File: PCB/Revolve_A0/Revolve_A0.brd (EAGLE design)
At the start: 100 x 100 mm, 386 parts, among them IC29 LAN8710A, IC30 MTFC2GMDEA, IC6 74AHC1G126DCK, IC7 74AHC1G126DCK, J2 4P-2.0, J3 4P-2.0, Q1 AON6758, Q10 DMC2038LVT, Q11 DMC2038LVT, Q13 DMC2038LVT, Q14 DMC2038LVT, Q2 AON6758, Q3 AON6758, Q8 AON6758, Q9 MMBT2907, U1 OSD3358-512M-BSM, U10 TPD4S012_DRY_6, U11 SN74AHC595PW, U13 INA199A1DCKR, U19 CD4050BD, U2 TUSB2046BIRHBT, U3 TPS2061D, U4 TPD4S012_DRY_6_P1_P, U5 UA78L05ACD, U6 TPD4S012_DRY_6_P1_P, U7 TLVH431, U8 TPD4S012_DRY_6_P1_P, U9 TPD4S012_DRY_6_P1_P, X1 22-05-7038-03, X10 22-05-7038-03, X11 22-05-7038-03, X12 22-05-7048-04, X13 22-05-7038-03, X14 22-05-7048-04, X15 22-05-7048-04, X16 22-05-7048-04, X17 22-05-7048-04, X18 22-05-7048-04, X19 22-05-7038-03, X2 MSTBA4, X20 MSTBA4, X21 MSTBA2, X22 22-05-7038-03, X24 HDMI4, X25 22-05-7048-04, X26 MSTBA2, X29 22-05-7038-03, X3 MSTBA2, X4 22-05-7028-02, X5 22-05-7028-02, X6 22-05-7028-02, X7 22-05-7038-03, X8 22-05-7038-03, X9 22-05-7028-02, Y1 25MHz, Y2 25MHz, Y4 6 MHz

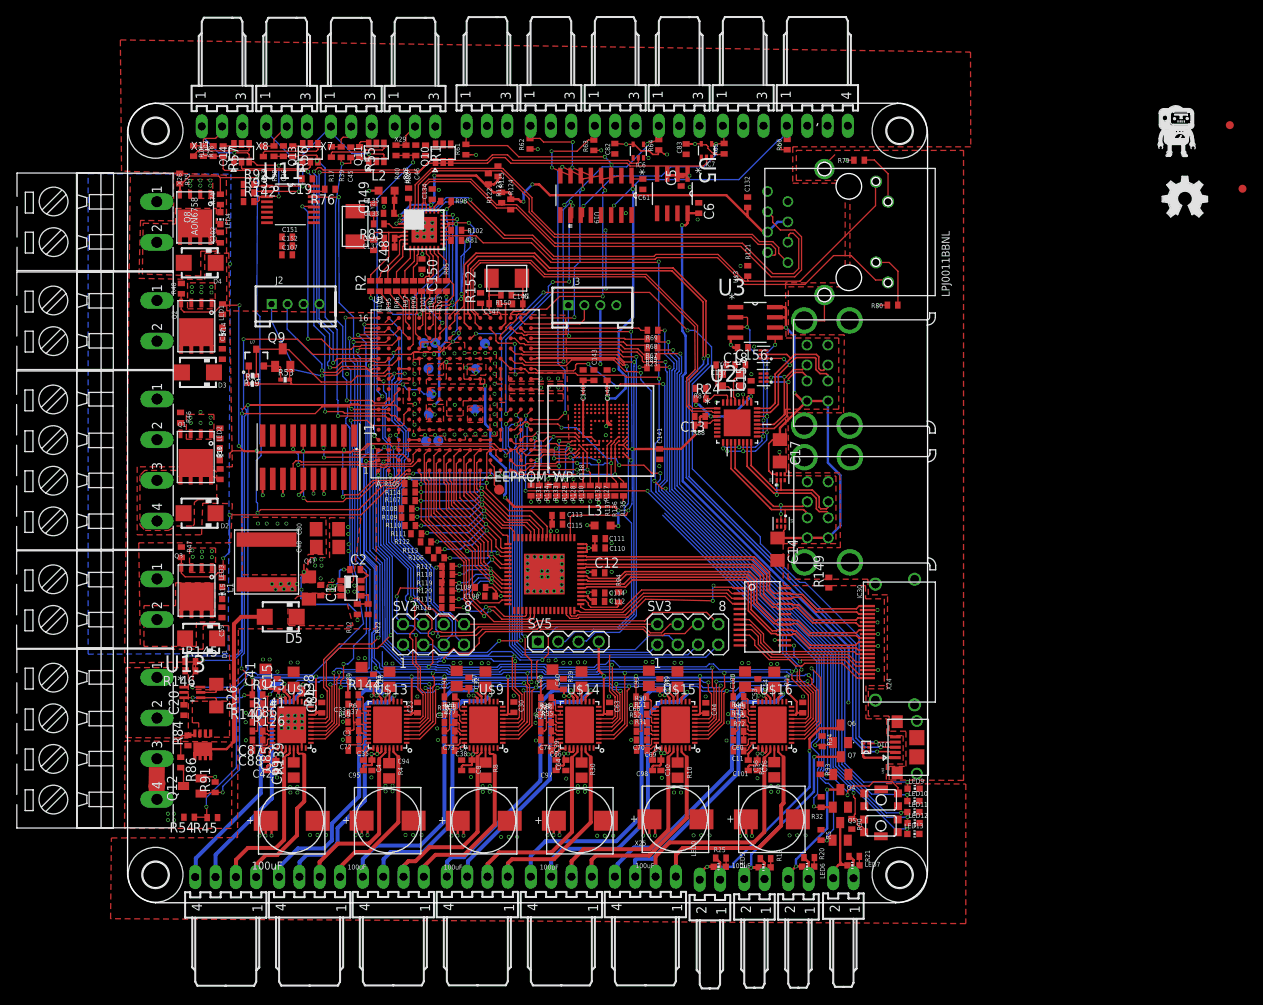
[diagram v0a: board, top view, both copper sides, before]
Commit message: Working on DRC errors
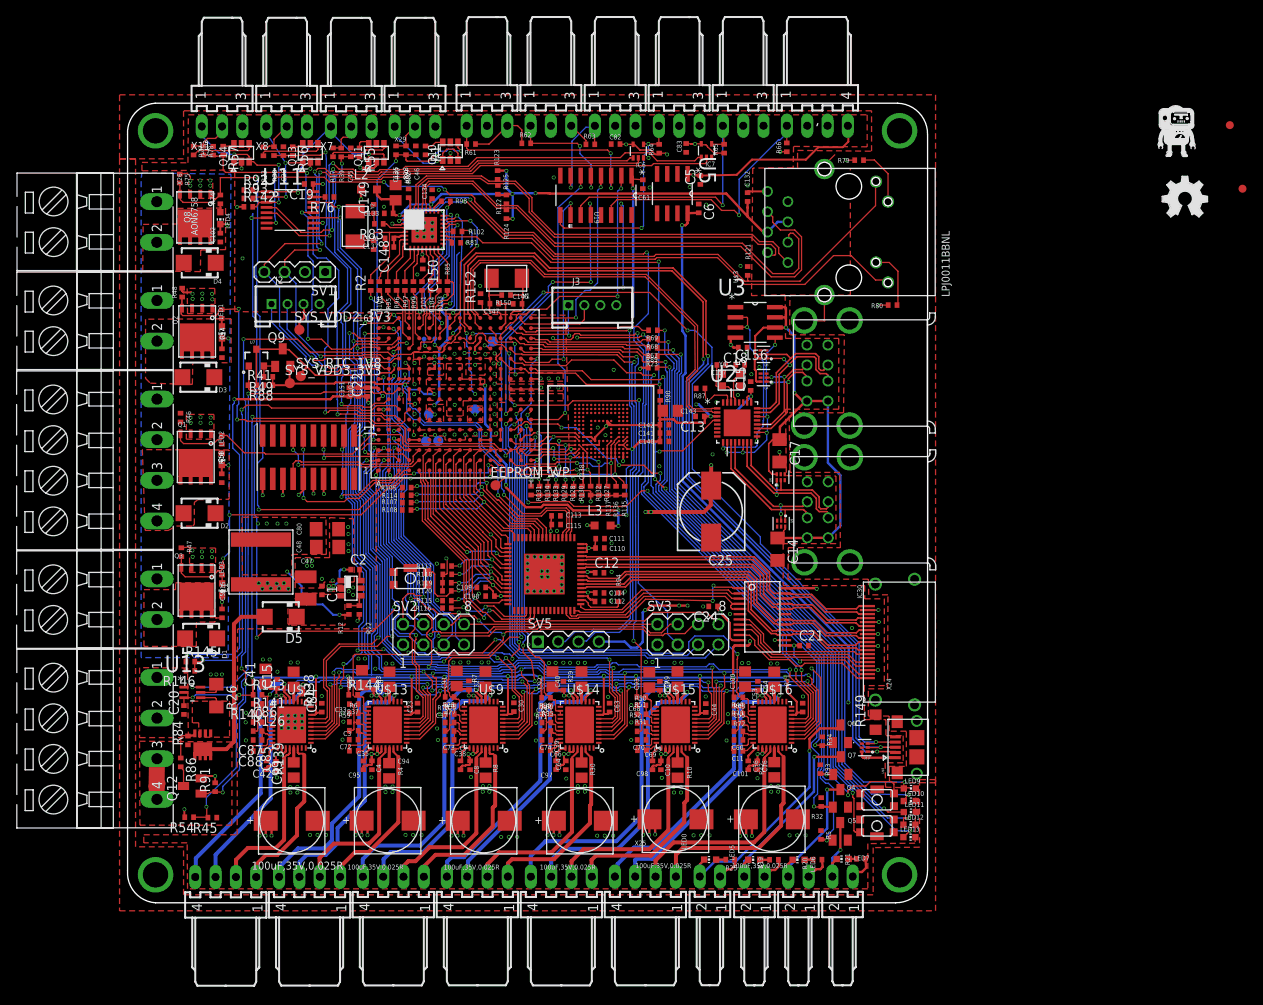
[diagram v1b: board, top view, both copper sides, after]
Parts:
- removed C152: 0.001uF, rcl:C0402
- removed H1, H2, H3, H4: MOUNT-HOLE3.2, holes:3,2
- removed R106, R109, R110, R111, R112, R113: 100K,1%, rcl:R0402
- removed R24: 0R,DNI, rcl:R0402
- removed R53: 499, OSD3358-SM-RED Platform:R0402
- added C21, C24: 0.1uF, rcl:C0402
- added C22: 4.7nF, rcl:C0402
- added C25: (no value), rcl:150CLZ-0810
- added MGT1, MGT2, MGT3, MGT4: MOUNTING_HOLE, OSD3358-SM-RED Platform:MOUNTING_HOLE
- added S1: KRM_TACT_SWITCH, Manga_custom:KMR
- added SV1: (no value), con-lstb:MA04-1
- C101, C42, C94, C95, C97, C98: value 100uF -> 100uF,35V,0.025R
- C132: value 0.022uF -> 22nF
- C135, C143: value 10uF -> 10uF,3.3V; device rcl:C0402 -> rcl:C0805
- C47: value 10uF -> 10uF,35V; device rcl:C1206 -> rcl:C1210
- L1: value 33uH -> 15uH
- R1, R121, R140, R141, R27, R31, R35, R37, R38, R39, R40, R43, R50, R55, R56, R57, R58, R6, R60, R73, R78, R81, R88: value 10K -> 10K,1%
- R122, R123, R124, R125: value 49.1, 1% -> 49.9,1%
- R127, R128, R129, R130, R131, R132, R133, R134, R135, R136, R137, R14, R142, R143, R144, R15, R16, R19, R20, R21, R23, R25, R28, R32, R33, R34, R36, R44, R46, R47, R48, R5, R51, R54, R61, R62, R63, R64, R65, R66, R67, R68, R69, R74, R75, R76, R87, R89, R91, R92, R93: value 4.7K -> 4.7K,1%
- R13, R17, R18, R77: value 4K7, 1% -> 4.7K,1%
- R149: value 0.1,5% -> 0.1R; device rcl:R0402 -> rcl:R0805
- R41: value 10K, 1% -> 40.2K,1%; device OSD3358-SM-RED Platform:R0402 -> rcl:R0402
- R49: value 40.2K, 1% -> 470; device OSD3358-SM-RED Platform:R0402 -> rcl:R0402
- R83: value 10 -> 10,1%
- SV2, SV3: value (none) -> DNI
- U10: value TPD4S012_DRY_6 -> TPD4S012_DRY_6_P1_P; device BeagleBone_Blue:DRY6 -> OSD3358-SM-RED Platform:DRY6
- VDDS_PLL, VDD_MPU: value TPB1,27 -> TPTP06R; device testpad:B1,27 -> testpad:TP06R
- moved R90 58.6 mm to (66.6, 63.4)
- moved R88 54.2 mm to (17.6, 64.7)
- moved SYS_RTC_1V8 21.9 mm to (21.7, 65.8), flipped to the top
- moved C151 20.9 mm to (27.7, 63.9), turned to 90 degrees
- moved C107 19.3 mm to (28.9, 63.9), turned to 90 degrees
- moved R149 18.4 mm to (93.5, 22.6)
- moved SYS_VDD3_3V3 17.7 mm to (20.3, 65.0), flipped to the top
- moved SYS_VDD2_3V3 16.9 mm to (21.5, 71.6), flipped to the top
- moved C140 13.1 mm to (67.1, 57.7), turned to 0 degrees
- moved C143 10.5 mm to (67.9, 61.5), turned to 0 degrees
- moved C142 9.47 mm to (67.1, 59.8), turned to 0 degrees
- moved C141 2.70 mm to (67.1, 58.7), turned to 0 degrees
- moved C5 2.40 mm to (71.6, 90.3)
- moved L2 2.21 mm to (30.2, 89.2)
- moved R49 2.01 mm to (17.6, 65.8)
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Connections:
- removed net FAULT_B: SV2.1, U1.T12
- removed net FAULT_C: SV3.1, U1.R5
- removed net PMIC_SCL: U1.C10, U1.D10
- removed net PMIC_SDA: U1.C11, U1.D11
- removed net TK_H: U1.C8
- removed net TRSRTN: J1.2
- removed net UNUSED_1: U1.J14
- removed net USB1_DRVVBUS: U1.M14
- removed net USB_RESET: R88.1, U2.4
- removed net VDD_3V3B: R90.1
- new net PMIC_MUX: U1.C8, U1.N13
- net +5V: no longer C18.2, C19.1, C82.1, C83.1, IC6.5, IC7.5, R61.2, R62.2, R63.2, R64.2, R65.2, R66.2, U$18.P$11, U11.10, U11.16, U3.4, X1.3, X10.3, X12.3, X13.3, X19.3, X22.3
- net CGND: now also MGT1.P$1, MGT2.P$1, MGT3.P$1, MGT4.P$1
- net CLKOUT2_48MHZ: no longer U2.27
- net DVI_+5V: now also C21.1
- net ENABLE_B: now also U11.6; no longer U1.T7
- net ENABLE_C: now also U11.7; no longer U1.R7
- net FAULT_A: now also U1.R5
- net FAULT_E: now also U1.T7
- net FAULT_H: now also U1.J14
- net FAULT_Y: now also U1.R7
- net FAULT_Z: now also U1.T12
- net GND: now also C21.2, C24.2, C25.-, R117.2, S1.2, SV1.1, SV2.1, SV3.1; no longer R106.1, R109.1, R110.1, R111.1, R112.1, R113.1
- net GNDA_ADC: now also C22.2; no longer C152.2
- net HDMI_HPD: now also U$18.P$5
- net I2C0_SCL: now also U1.C10, U1.D10
- net I2C0_SDA: now also U1.C11, U1.D11
- net LCD_D10: no longer R110.2
- net LCD_D11: no longer R109.2
- net LCD_D2: now also S1.1
- net LCD_D6: no longer R106.2
- net LCD_D7: no longer R113.2
- net LCD_D8: no longer R112.2
- net LCD_D9: no longer R111.2
- net N$1: now also R88.2; no longer R49.2
- net N$192: no longer R24.2
- net N$4: now also R49.2; no longer R53.1
- net SERVO_0: now also SV1.3
- net SERVO_1: now also SV1.4
- net SYS_5V: now also C18.2, C19.1, C24.1, C25.+, C82.1, C83.1, IC6.5, IC7.5, R61.2, R62.2, R63.2, R64.2, R65.2, R66.2, U$18.P$11, U11.10, U11.16, U3.4, X1.3, X10.3, X12.3, X13.3, X19.3, X22.3
- net SYS_RESETN: now also U2.4
- net SYS_RTC_1V8: now also R41.2; no longer R49.1
- net SYS_VDD1_3V3: now also R90.1, U$18.P$12; no longer R117.2, R24.1, R88.2, SV5.4
- net SYS_VDD2_3V3: now also SV1.2, SV5.4
- net SYS_VDD3_3V3: now also R49.1, R88.1; no longer R41.2, R53.2
- net TRSTN: now also J1.2
- net USB0_DM: now also U10.1; no longer U10.2
- net USB0_DP: now also U10.2; no longer U10.1
- net VDD_ADC: now also C22.1; no longer C152.1
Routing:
- net FAULT_B: track 90.1 -> 0.00 mm, vias 3 -> 0
- net FAULT_H: track 4.22 -> 73.9 mm, vias 0 -> 4
- net SERVO_1_EN: track 0.00 -> 66.6 mm, vias 0 -> 2
- net FAULT_A: track 3.80 -> 68.0 mm, vias 0 -> 2
- net ENABLE_C: track 51.5 -> 110.6 mm, vias 1 -> 5
- net FAULT_Y: track 3.48 -> 62.4 mm, vias 0 -> 4
- net STEP_A: track 37.3 -> 95.9 mm, vias 1 -> 4
- net SPI0_MISO: track 36.8 -> 94.0 mm, vias 1 -> 4
- net SERVO_0_EN: track 0.00 -> 56.1 mm, vias 0 -> 2
- net CLKOUT2_48MHZ: track 53.4 -> 0.00 mm, vias 2 -> 0
- net DIR_E: track 10.1 -> 63.1 mm, vias 0 -> 4
- net FAULT_Z: track 3.12 -> 55.5 mm, vias 0 -> 2
- net SYS_5V: track 0.64 -> 51.4 mm, vias 1 -> 12
- net FAULT_C: track 45.8 -> 0.00 mm, vias 1 -> 0
- net I2C0_SDA: track 0.00 -> 41.3 mm, vias 0 -> 2
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- added copper zone on layer 1, net N$64
- added copper zone on layer 3, net SYS_5V
- added copper zone on layer 3, net SYS_VDD2_3V3
- removed copper zone on layer 3, net +12V
- removed copper zone on layer 1, net +24V
- removed copper zone on layer 3, net N$42
